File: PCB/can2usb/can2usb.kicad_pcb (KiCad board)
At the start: 2 copper layers, 36 parts, among them J1 STLINK, J2 Conn_01x03_Male, P1 USB_C_Plug_USB2.0, SW1 BOOT_SW, U1 STM32F103C6Tx, U2 TLP175A, U3 MCP2561-E-SN, U4 LM1117-3.3, U5 USBLC6-2SC6, Y1 16MHz, Y2 32KHz

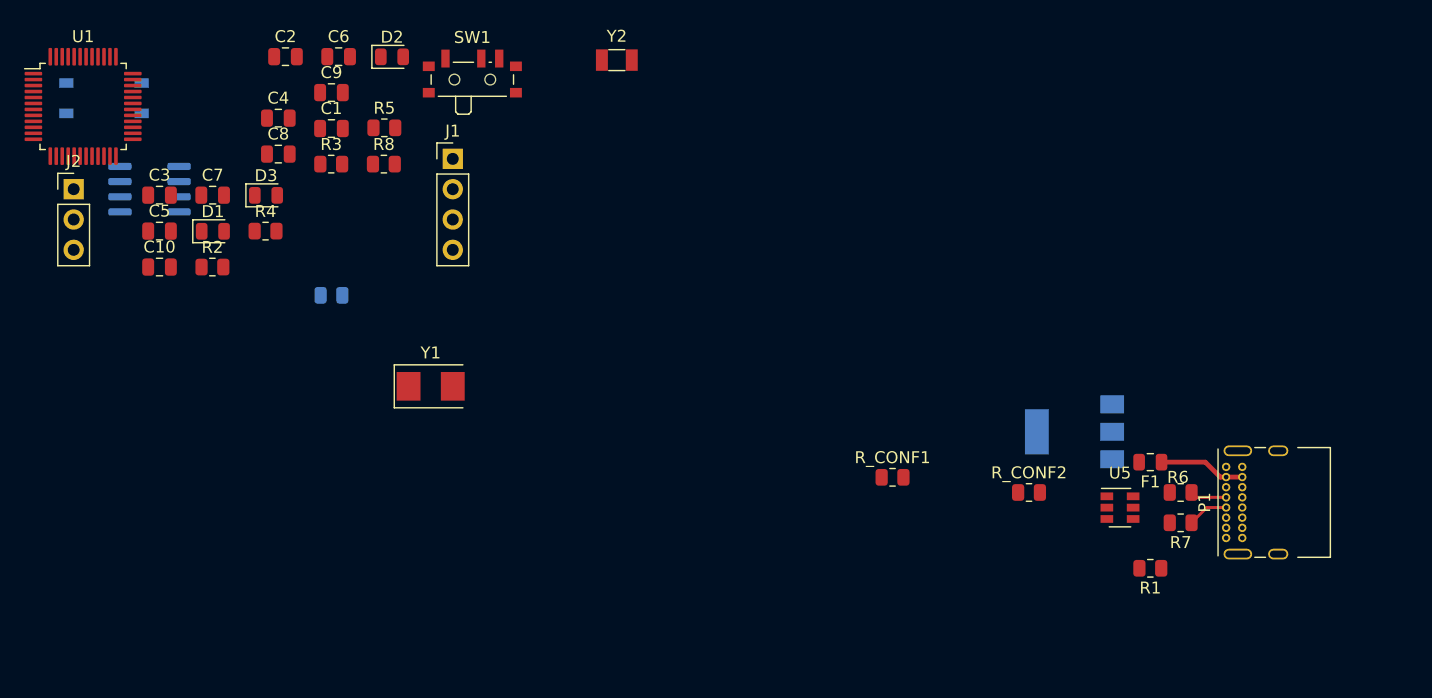
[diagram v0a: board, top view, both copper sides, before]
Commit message: First version pcb
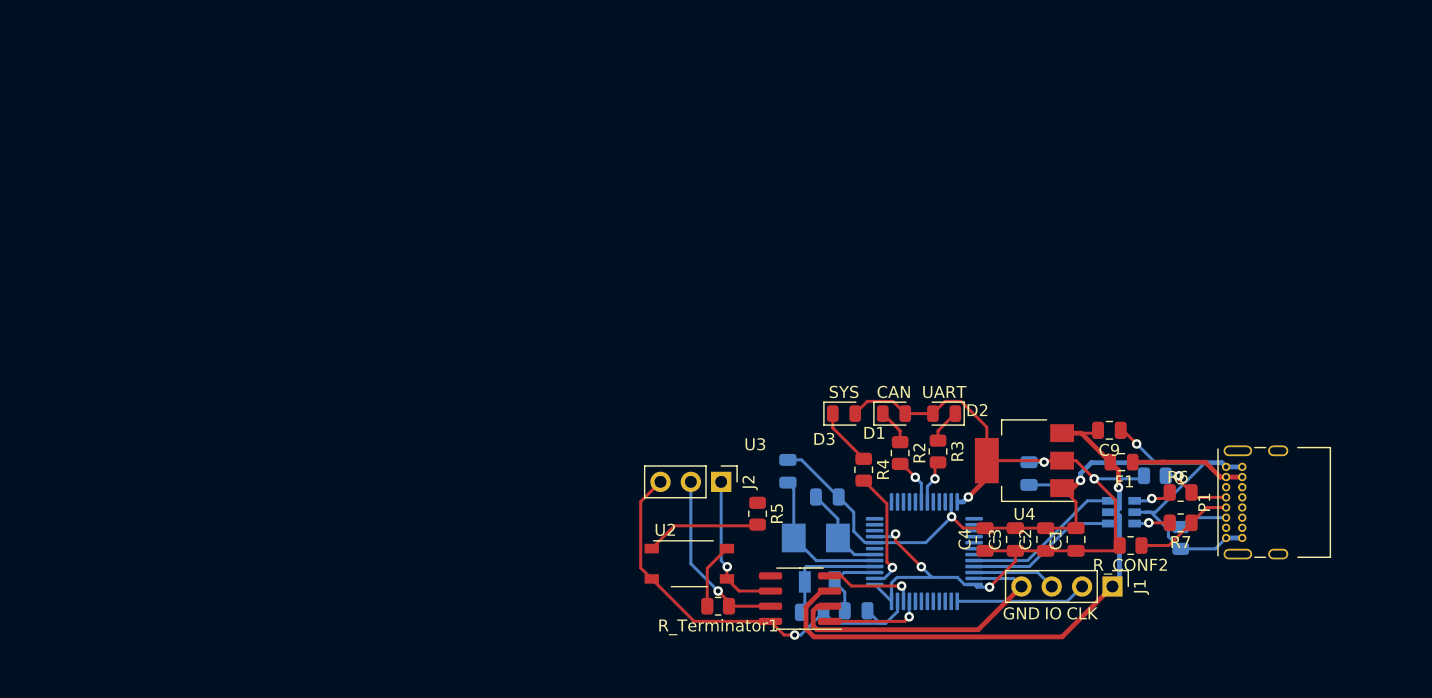
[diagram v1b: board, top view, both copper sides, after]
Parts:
- removed R8: 1k, Resistor_SMD:R_0805_2012Metric
- removed SW1: BOOT_SW, Button_Switch_SMD:SW_SPDT_PCM12
- C10, C5, C6, C7, C8, R1, R_CONF1, U1, U5, Y1, Y2: moved to B.Cu
- R_Terminator1, U2, U3, U4: moved to F.Cu
- moved U1 79.7 mm to (89.0, 58.3)
- moved C3 77.3 mm to (96.6, 57.3), turned to 90 degrees
- moved C2 75.4 mm to (99.2, 57.3), turned to 90 degrees
- moved C10 74.8 mm to (97.8, 51.8), turned to 90 degrees
- moved C1 71.2 mm to (101.7, 57.3), turned to 90 degrees
- moved C9 71.0 mm to (104.5, 48.1), turned to 180 degrees
- moved C4 68.9 mm to (94.1, 57.3), turned to 90 degrees
- moved J1 65.8 mm to (104.8, 61.2), turned to 270 degrees
- moved U3 64.4 mm to (78.6, 62.2), turned to 180 degrees
- moved C7 64.2 mm to (83.3, 63.2)
- moved U2 62.6 mm to (69.3, 59.3)
- moved R2 59.7 mm to (87.0, 50.0), turned to 270 degrees
- moved J2 59.5 mm to (72.0, 52.5), turned to 270 degrees
- moved D1 59.1 mm to (86.5, 46.7)
- moved C8 58.9 mm to (79.6, 63.4)
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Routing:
- net GND: track 0.00 -> 140.0 mm, vias 0 -> 4
- net +3V3: track 0.00 -> 77.0 mm, vias 0 -> 6
- net +5V: track 0.00 -> 50.5 mm, vias 0 -> 1
- net CAN_H: track 0.00 -> 15.2 mm, vias 0 -> 1
- net USB_D-: track 0.00 -> 13.3 mm
- net USB_D+: track 0.00 -> 12.7 mm
- net CAN_L: track 0.00 -> 12.4 mm, vias 0 -> 1
- net OSC_IN: track 0.00 -> 12.4 mm
- net SWCLK: track 0.00 -> 11.0 mm
- net B_LED: track 0.00 -> 10.5 mm, vias 0 -> 1
- net L_OSC_OUT: track 0.00 -> 10.1 mm
- net Net-(R5-Pad2): track 0.00 -> 9.70 mm
- net OSC_OUT: track 0.00 -> 8.65 mm
- net CAN_RX: track 0.00 -> 8.13 mm, vias 0 -> 1
- net CAN_TX: track 0.00 -> 7.73 mm, vias 0 -> 1
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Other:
- board text added: "CAN"
- board text added: "CLK"
- board text added: "GND"
- board text added: "IO"
- board text added: "SYS"
- board text added: "UART"

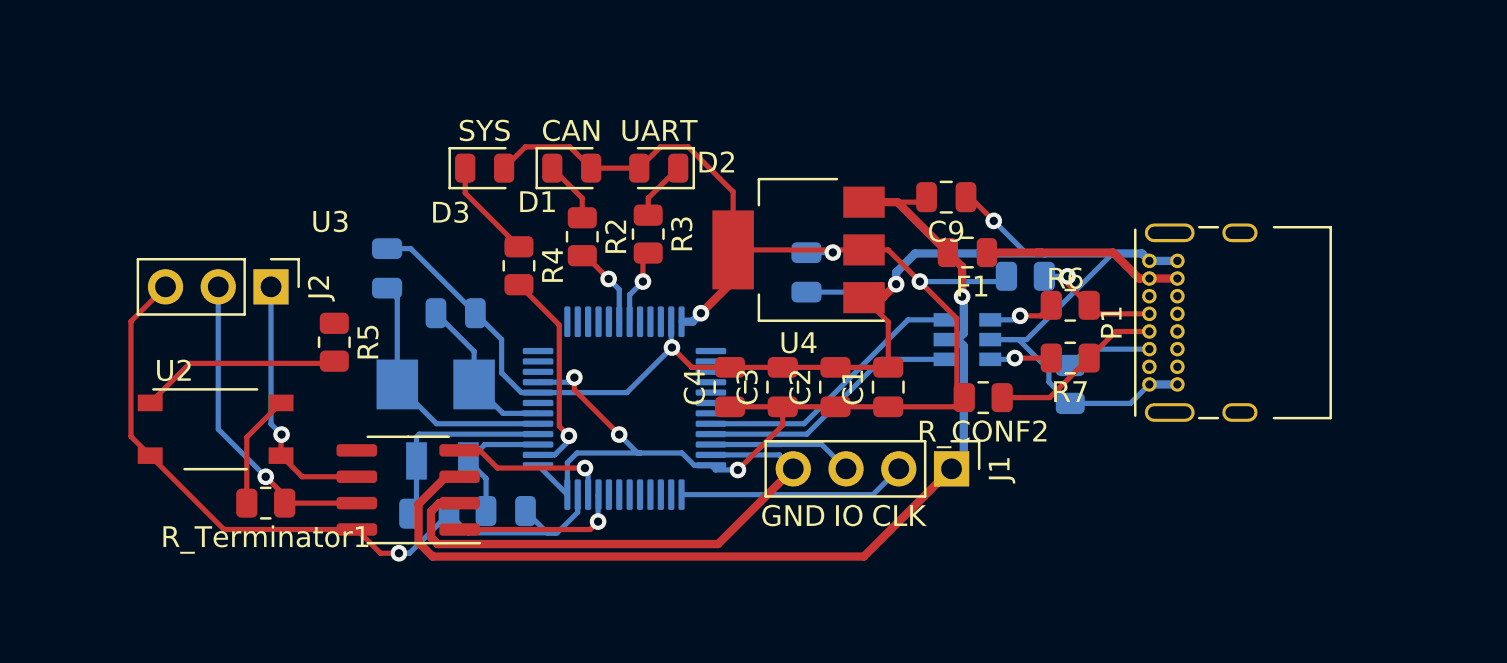
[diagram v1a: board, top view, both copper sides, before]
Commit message: Finished brd
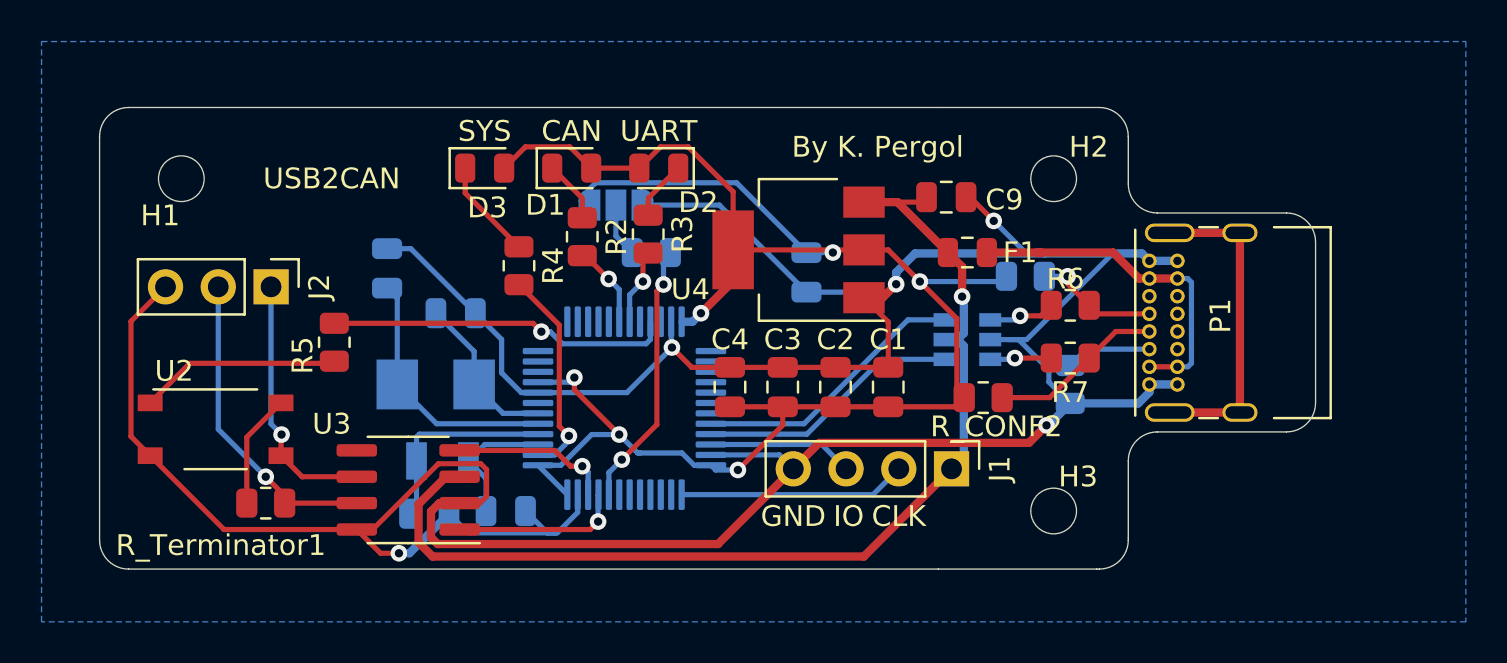
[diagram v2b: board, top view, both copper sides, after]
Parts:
- added H1: MountingHole, MountingHole:MountingHole_2.2mm_M2, F.Cu at (67.7, 47.2)
- added H2: MountingHole, MountingHole:MountingHole_2.2mm_M2, F.Cu at (109.7, 47.2)
- added H3: MountingHole, MountingHole:MountingHole_2.2mm_M2, F.Cu at (109.7, 63.2)
- added JP1: SolderJumper_3_Open, Jumper:SolderJumper-3_P1.3mm_Open_RoundedPad1.0x1.5mm, B.Cu at (88.6, 48.5)
- added R8: 1k, Resistor_SMD:R_0805_2012Metric, B.Cu at (90.3, 50.8)
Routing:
- net GND: track 140.0 -> 174.9 mm, vias 4 -> 5
- net TERMINATOR_SW: track 0.00 -> 16.6 mm, vias 0 -> 1
- net Net-(P1-PadS1): track 0.00 -> 15.4 mm
- net BOOT0: track 0.00 -> 12.9 mm, vias 0 -> 2
- net +3V3: track 77.0 -> 89.1 mm
- net Net-(F1-Pad1): track 9.90 -> 16.6 mm
- net Net-(JP1-Pad2): track 0.00 -> 2.61 mm
- added copper zone on B.Cu, net GND
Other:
- board outline added: 58.5 x 22.2 mm
- board text added: "By K. Pergol"
- board text added: "By Karol Pergol"
- board text added: "USB2CAN"
